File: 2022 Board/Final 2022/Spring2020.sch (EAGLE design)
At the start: 23 parts, among them U1 TB67H401FTG(O,EL), U2 ABX00012

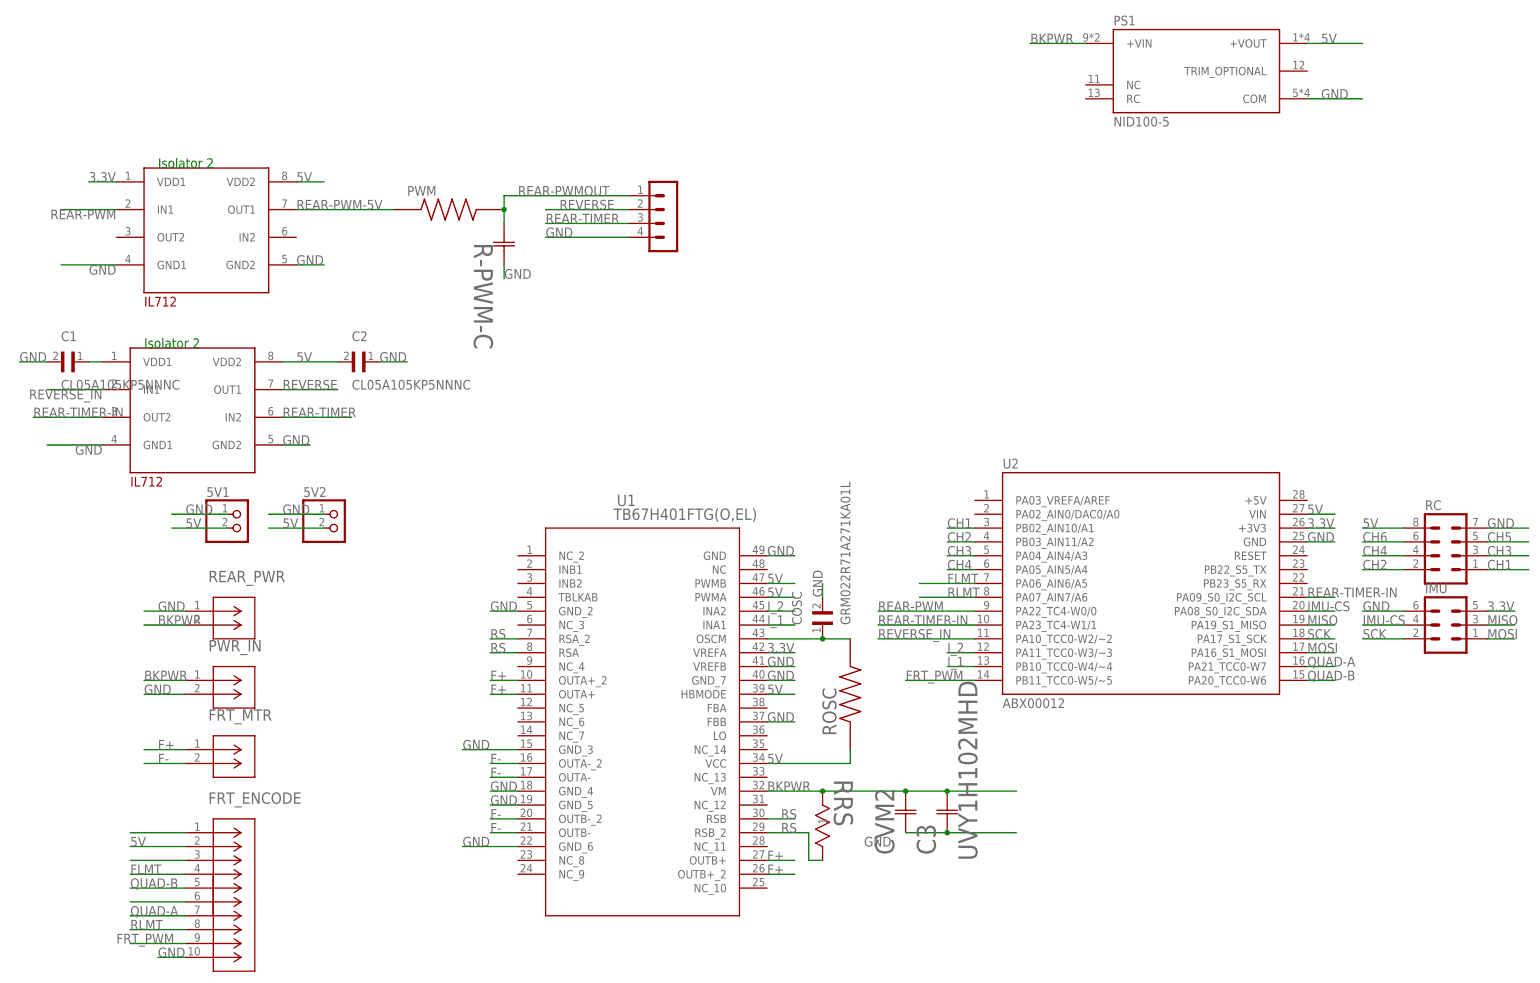
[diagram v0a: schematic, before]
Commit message: Just a few random edits
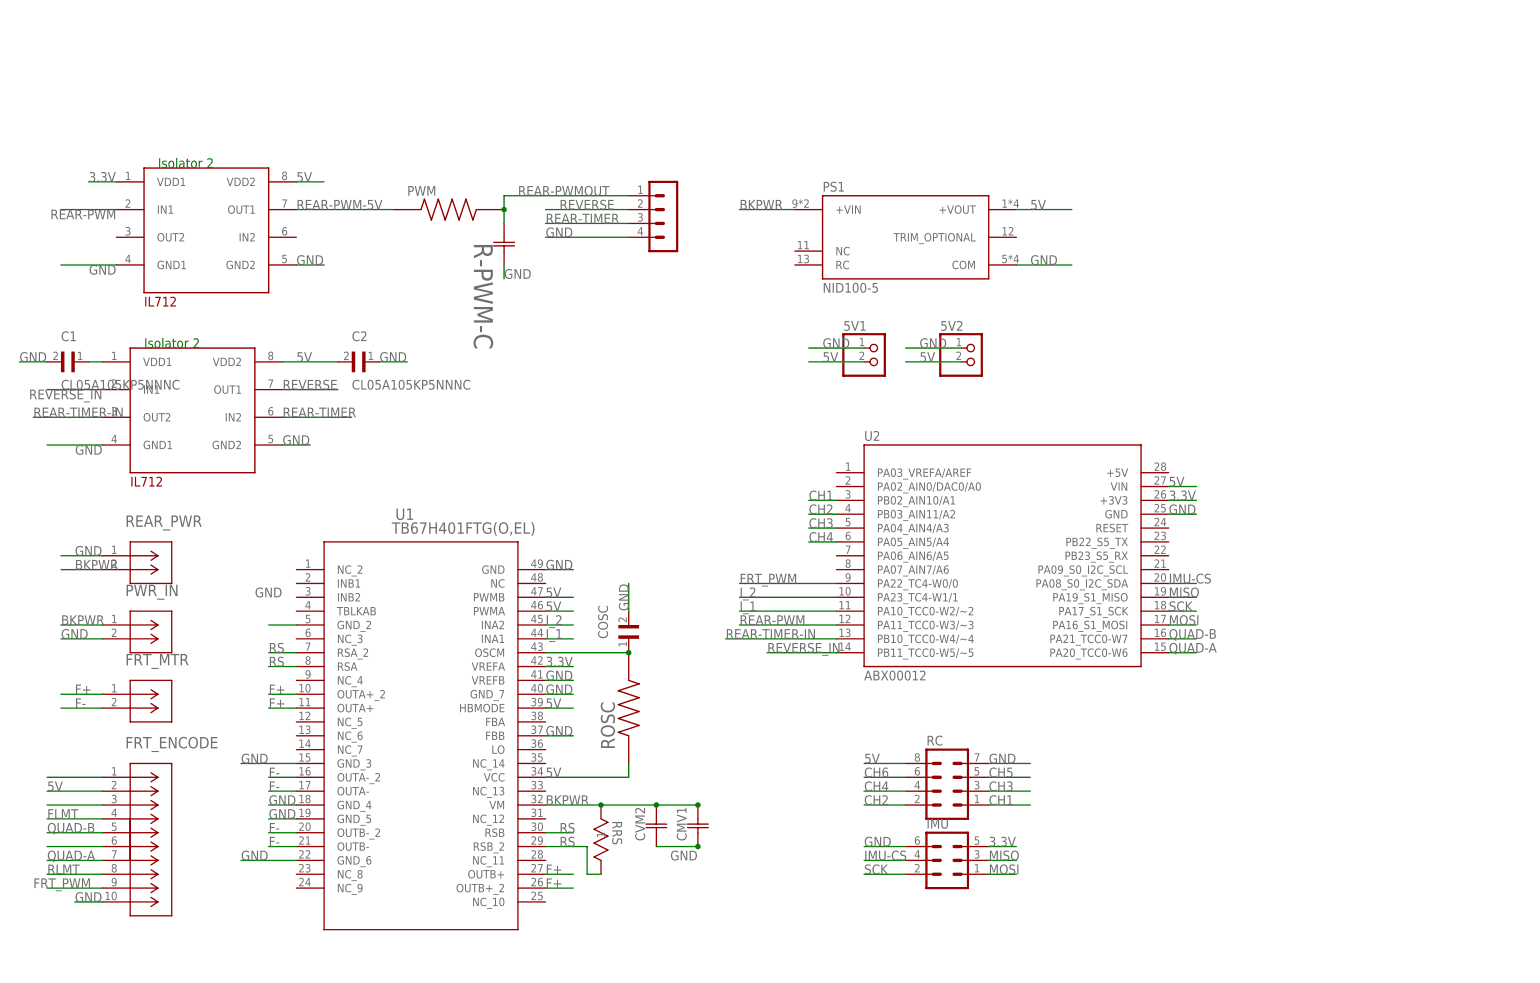
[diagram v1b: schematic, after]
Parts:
- removed C3: UVY1H102MHD, Test2:UVY1H102MHD
- added CMV1: UVY1H102MHD, Test2:UVY1H102MHD
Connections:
- net BKPWR: now also CMV1.2; no longer C3.2
- net FLMT: no longer U2.PA06_AIN6/A5
- net FRT_PWM: now also U2.PA22_TC4-W0/0; no longer U2.PB11_TCC0-W5/~5
- net GND: now also CMV1.1; no longer C3.1
- net I_1: now also U2.PA10_TCC0-W2/~2; no longer U2.PB10_TCC0-W4/~4
- net I_2: now also U2.PA23_TC4-W1/1; no longer U2.PA11_TCC0-W3/~3
- net QUAD-A: now also U2.PA20_TCC0-W6; no longer U2.PA21_TCC0-W7
- net QUAD-B: now also U2.PA21_TCC0-W7; no longer U2.PA20_TCC0-W6
- net REAR-PWM: now also U2.PA11_TCC0-W3/~3; no longer U2.PA22_TC4-W0/0
- net REAR-TIMER-IN: now also U2.PB10_TCC0-W4/~4; no longer U2.PA09_S0_I2C_SCL, U2.PA23_TC4-W1/1
- net REVERSE_IN: now also U2.PB11_TCC0-W5/~5; no longer U2.PA10_TCC0-W2/~2
- net RLMT: no longer U2.PA07_AIN7/A6
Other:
- moved on the sheet: 5V1, 5V2, COSC, CVM2, FRT_ENCODE, FRT_MTR, IMU, PS1, PWR_IN, RC, REAR_PWR, ROSC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
